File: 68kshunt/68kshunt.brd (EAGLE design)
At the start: 113 x 39.4 mm, 2 parts

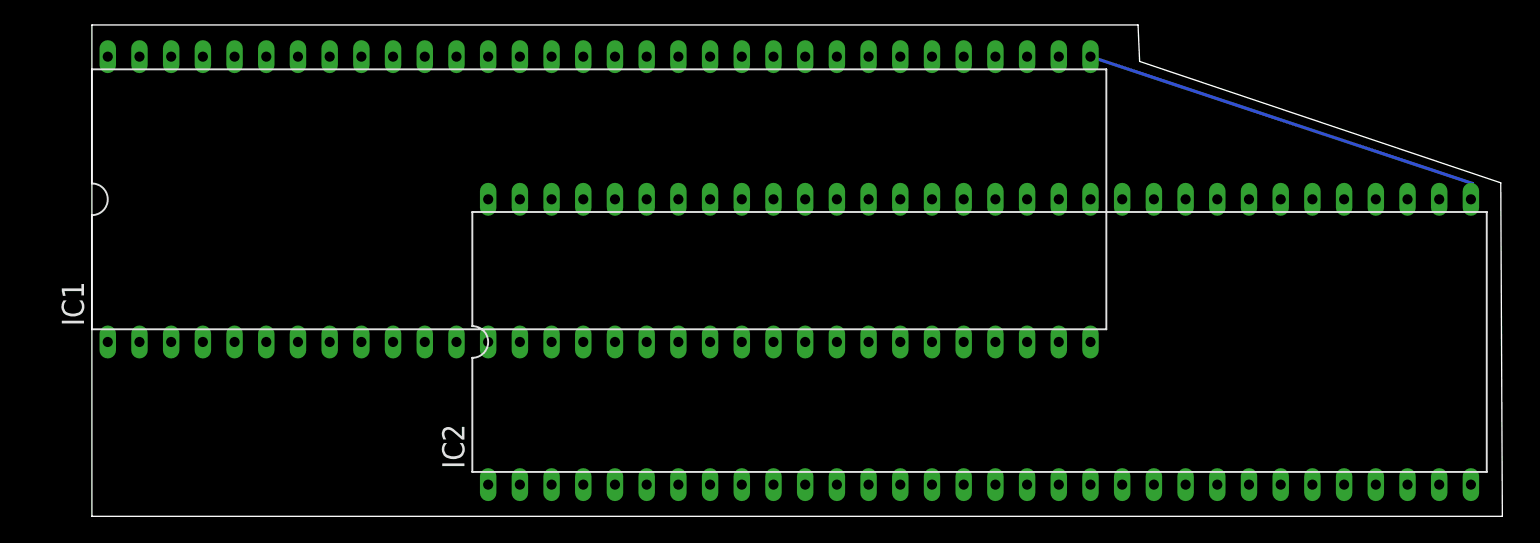
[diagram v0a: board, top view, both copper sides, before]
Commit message: Ok I routed this... :(
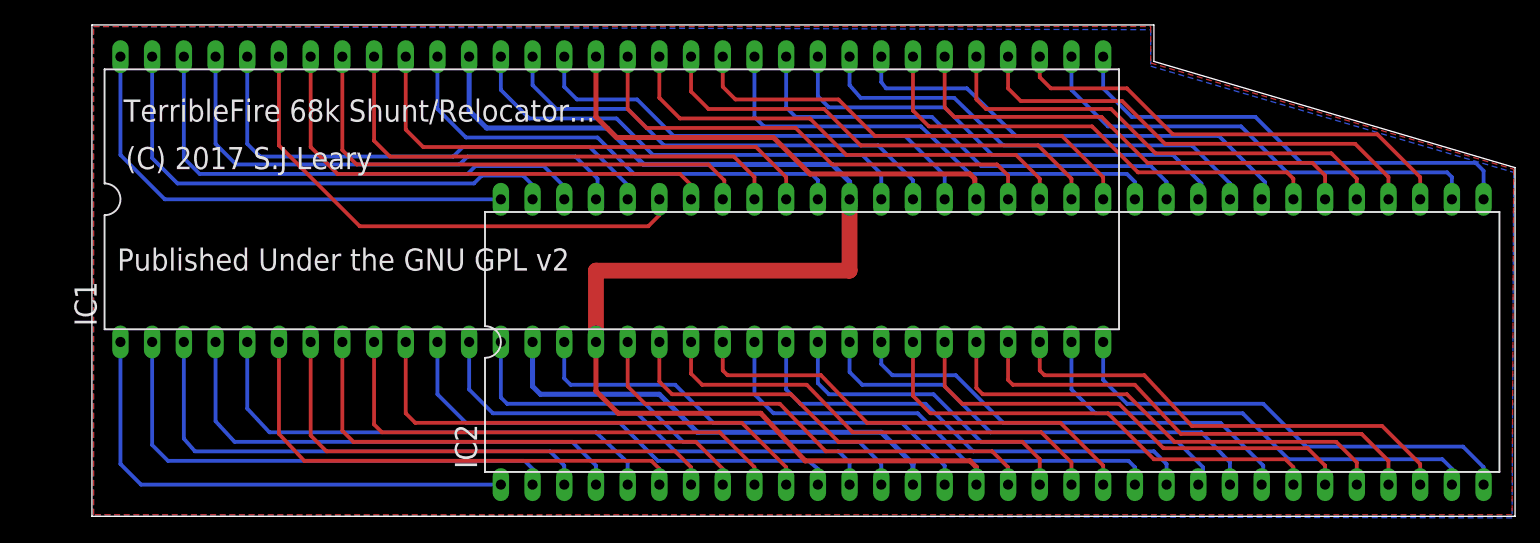
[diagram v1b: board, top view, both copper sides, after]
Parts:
- moved IC1 1.02 mm to (41.7, 25.4)
- moved IC2 1.02 mm to (72.1, 14.0)
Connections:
- removed net GND1: IC1.16, IC2.16
- removed net GND2: IC1.53, IC2.53
- removed net VCC1: IC1.14, IC2.14
- removed net VCC2: IC1.49, IC2.49
- new net GND: IC1.16, IC1.53, IC2.16, IC2.53
- new net VCC: IC1.14, IC1.49, IC2.14, IC2.49
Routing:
- net GND: track 0.00 -> 108.7 mm
- net VCC: track 0.00 -> 77.2 mm
- net D10: track 0.00 -> 41.9 mm
- net D6: track 0.00 -> 41.5 mm
- net D7: track 0.00 -> 41.3 mm
- net D8: track 0.00 -> 41.0 mm
- net D4: track 0.00 -> 40.9 mm
- net D3: track 0.00 -> 40.9 mm
- net D2: track 0.00 -> 40.7 mm
- net D12: track 0.00 -> 40.7 mm
- net D9: track 0.00 -> 40.6 mm
- net UDS: track 0.00 -> 40.4 mm
- net AS: track 0.00 -> 40.3 mm
- net D11: track 0.00 -> 40.2 mm
- net D13: track 0.00 -> 40.2 mm
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- added copper zone on layer 1, net GND
- added copper zone on layer 16, net VCC
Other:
- board size 113 x 39.4 mm -> 114 x 39.4 mm
- board text added: "(C) 2017 S.J Leary"
- board text added: "Published Under the GNU GPL v2"
- board text added: "TerribleFire 68k Shunt/Relocator..."

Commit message: Updates to the board files.
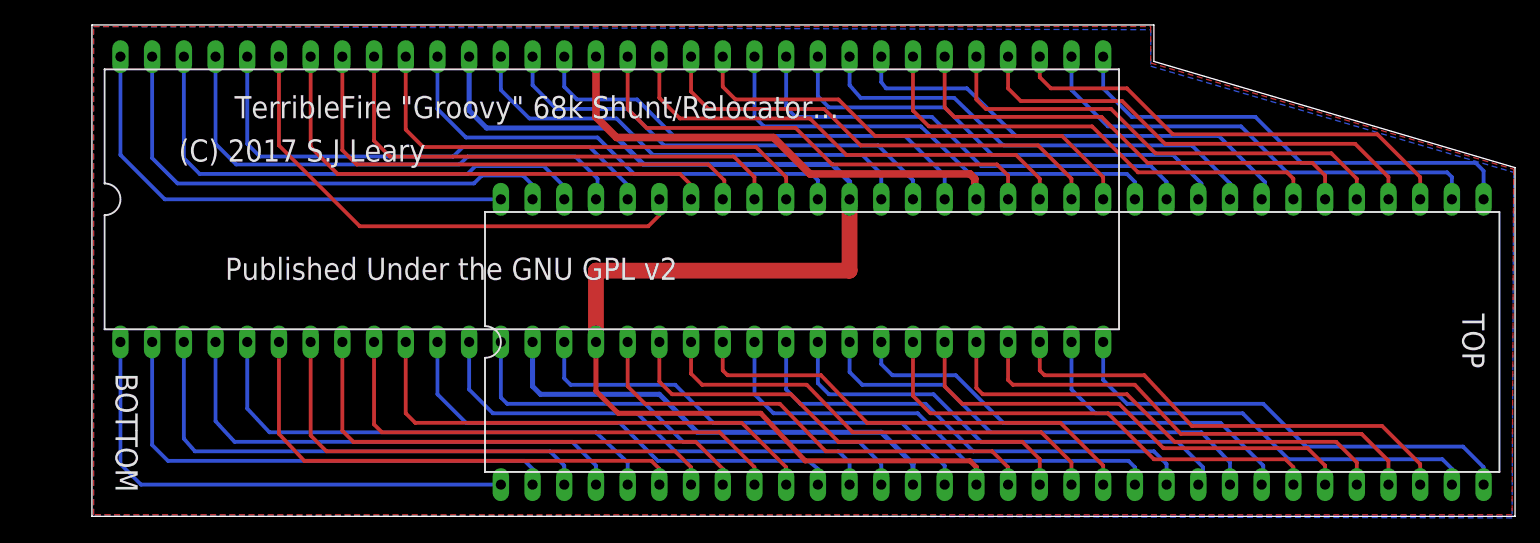
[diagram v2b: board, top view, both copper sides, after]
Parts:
- renumbered IC1 to BOTTOM, IC2 to TOP
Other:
- board text added: "C:/Users/stephen/Downloads/bwlogo.bmp"
- board text added: "TerribleFire "Groovy" 68k Shunt/Relocator..."
- board text removed: "TerribleFire 68k Shunt/Relocator..."
